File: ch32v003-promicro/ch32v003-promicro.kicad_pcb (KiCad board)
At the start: 2 copper layers, 17.8 x 33 mm, 24 parts, among them J1 USB2.0_C_v3, J2 ProMicro-LeftPin, J3 ProMicro-RightPin, SW1 SW_Push, U1 CH32V003F4P6, U2 AMS1117-3.3, Y1 24M

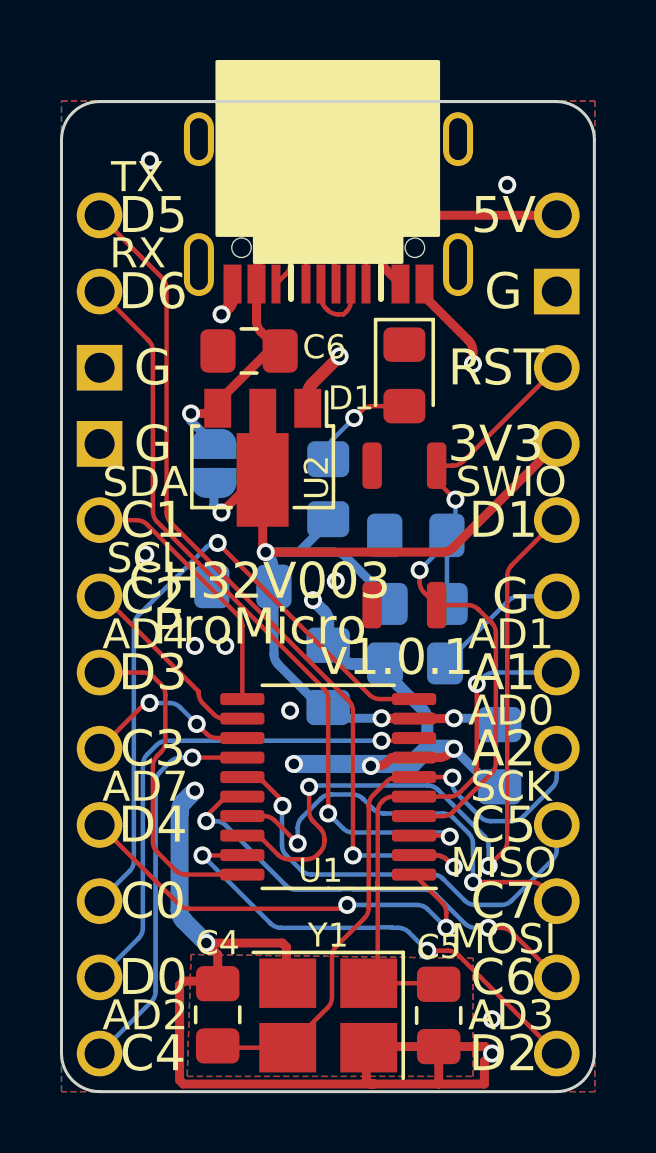
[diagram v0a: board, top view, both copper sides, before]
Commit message: ch32v003promicro/1.1.0
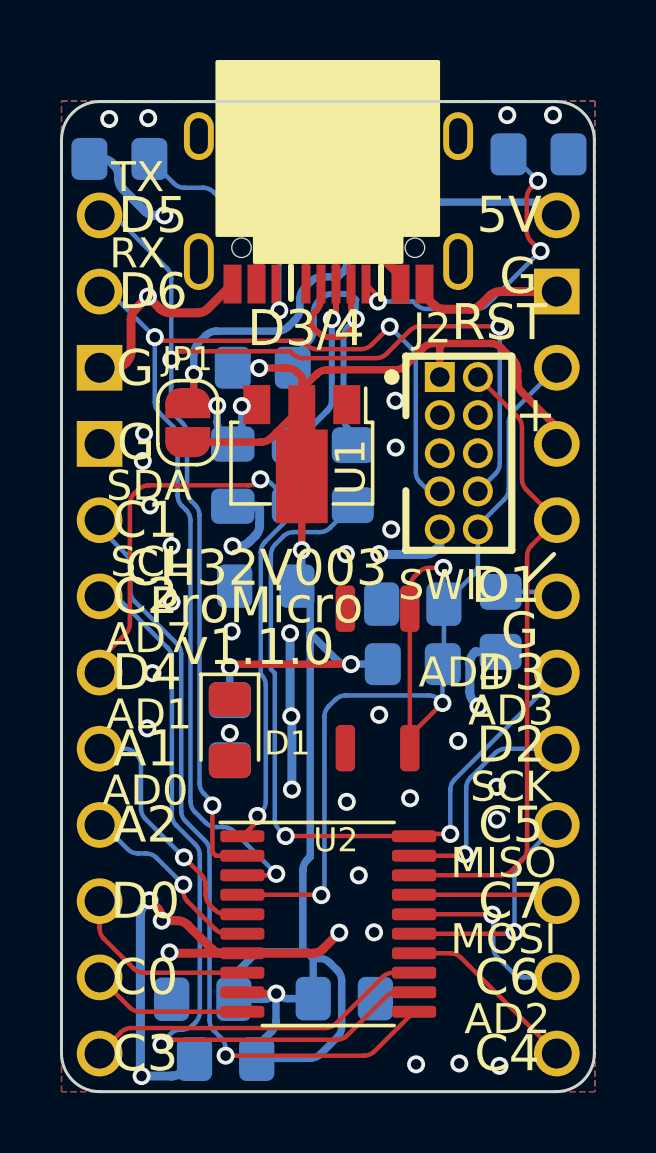
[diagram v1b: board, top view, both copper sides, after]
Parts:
- removed the C4 at (103.0, 92.7)
- removed the C5 at (110.4, 92.7)
- removed the REF** at (104.1, 93.2)
- removed Y1: 24M, $74th:Crystal_SMD_3225-4Pin_3.2x2.5mm_HandSoldering
- added C6: 1u, $74th:Capacitor_0805_2012, B.Cu at (103.3, 94.2)
- added J2: SWD-MCU_Side-10Pin, $74th:SWD_2x05_P1.27mm, F.Cu at (110.4, 71.4)
- added MISC-ACCOUNTTEXT: 74th-text, $74th:74th-text, B.Cu at (111.5, 88.9)
- added MISC-ACCOUNTTEXT: 74th-text, $74th:74th-text, B.Cu at (110.2, 88.8)
- added R1: 10k, $74th:Register_0805_2012, B.Cu at (108.6, 63.2)
- added R2: 54k, $74th:Register_0805_2012, B.Cu at (104.8, 63.2)
- added R5: 1.5k(NC), $74th:Register_0805_2012, B.Cu at (104.5, 71.1)
- added R6: 27.4(NC), $74th:Register_0805_2012, B.Cu at (107.5, 74.7)
- added R7: 27.4(NC), $74th:Register_0805_2012, B.Cu at (105.5, 74.7)
- added U3: CH217K, Package_TO_SOT_SMD:SOT-23-6, B.Cu at (107.1, 65.9)
- C1: renamed from C6; moved to B.Cu
- C2: renamed from C7; value 2.2u -> 10u
- JP1: moved to F.Cu
- R10: renamed from R4; value 200 -> 10k
- moved REF** 18.2 mm to (100.7, 83.2)
- moved D1 13.2 mm to (103.4, 83.2)
- moved C5 12.8 mm to (102.5, 92.2), turned to 180 degrees
- moved C4 10.8 mm to (107.2, 92.2), turned to 0 degrees
- moved R10 8.68 mm to (103.4, 83.2), turned to -90 degrees
- moved G*** 7.45 mm to (110.4, 86.0)
- moved R3 6.04 mm to (113.7, 64.0), turned to 0 degrees
- moved R4 4.97 mm to (99.7, 64.2), turned to 180 degrees
- moved SW1 4.85 mm to (108.3, 81.5)
- moved U2 4.57 mm to (106.7, 89.7), turned to 0 degrees
- moved C1 4.17 mm to (103.5, 74.7), turned to -90 degrees
- moved R8 3.17 mm to (112.4, 79.6), turned to -90 degrees
- moved C3 2.29 mm to (109.5, 79.0)
- moved R9 2.02 mm to (109.5, 81.0)
- moved JP1 1.61 mm to (102.0, 73.0)
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- renumbered C1 to C3, C2 to C4, C3 to C5, J2 to J3, J3 to J4, R2 to R4, R5 to R8, R1 to R9, U2 to U1, U1 to U2
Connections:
- net 0/UART_RX renamed /0/UART_RX
- net 14/SPI_MISO renamed /14/SPI_MISO
- net 15/SPI_SCK renamed /15/SPI_SCK
- net 16/SPI_MOSI renamed /16/SPL_MOSI
- net 1/UART_TX renamed /1/UART_TX
- net 20/A2 renamed /20/A2
- net 21/A3 renamed /21/A3
- net 2/I2C_SDA renamed /2/I2C_SDA
- net 3/I2C_SCL renamed /3/I2C_SCL
- net RST renamed /RST
- J1 pad 1: +5V -> Net-(J1-VBUS)
- J1 pad 2: unconnected-(J1-D--Pad2) -> /USB_D-
- J1 pad 3: unconnected-(J1-D+-Pad3) -> /USB_D+
- J3 pad 10: 7 -> /7
- J3 pad 11: 8/A8 -> /8/A8
- J3 pad 12: 9/A9 -> /9/A9
- J3 pad 7: 4/A6 -> /4/A6
- J3 pad 8: 5 -> /5
- J3 pad 9: 6/A7 -> /6/A7
- J4 pad 1: 10/A10 -> /10/A10
- J4 pad 5: 18/A0 -> /18/A0
- J4 pad 6: 19/A1 -> /19/A1
- U2 pad 1: 6/A7 -> /4/A6
- U2 pad 10: 7 -> /8/A8
- U2 pad 13: 5 -> /9/A9
- U2 pad 14: 9/A9 -> /10/A10
- U2 pad 19: 10/A10 -> /18/A0
- U2 pad 20: 4/A6 -> /19/A1
- U2 pad 5: 19/A1 -> /5
- U2 pad 6: 18/A0 -> /6/A7
- U2 pad 8: 8/A8 -> /7
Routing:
- net /19/A1: track 0.00 -> 25.1 mm, vias 0 -> 2
- net VCC: track 38.8 -> 62.4 mm, vias 4 -> 5
- net /4/A6: track 0.00 -> 23.2 mm, vias 0 -> 2
- net 7: track 22.3 -> 0.00 mm, vias 1 -> 0
- net 18/A0: track 20.6 -> 0.00 mm, vias 1 -> 0
- net /3/I2C_SCL: track 6.55 -> 25.8 mm, vias 0 -> 1
- net 19/A1: track 18.6 -> 0.00 mm, vias 1 -> 0
- net /2/I2C_SDA: track 8.73 -> 26.0 mm, vias 0 -> 1
- net 8/A8: track 17.1 -> 0.00 mm, vias 1 -> 0
- net 10/A10: track 15.8 -> 0.00 mm, vias 2 -> 0
- net 6/A7: track 15.2 -> 0.00 mm, vias 2 -> 0
- net /USB_D-: track 0.00 -> 13.2 mm, vias 0 -> 1
- net 9/A9: track 13.1 -> 0.00 mm, vias 1 -> 0
- net /RST: track 23.5 -> 35.1 mm, vias 2 -> 3
- net /9/A9: track 0.00 -> 11.5 mm
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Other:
- board text added: "+"
- board text added: "D3/4"
- board text added: "USB"
- board text added: "v1.1.0"
- board text removed: "3V3"
- board text removed: "v1.0.0"
- board text removed: "v1.0.1"

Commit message: ch32v003promicro/1.2.0
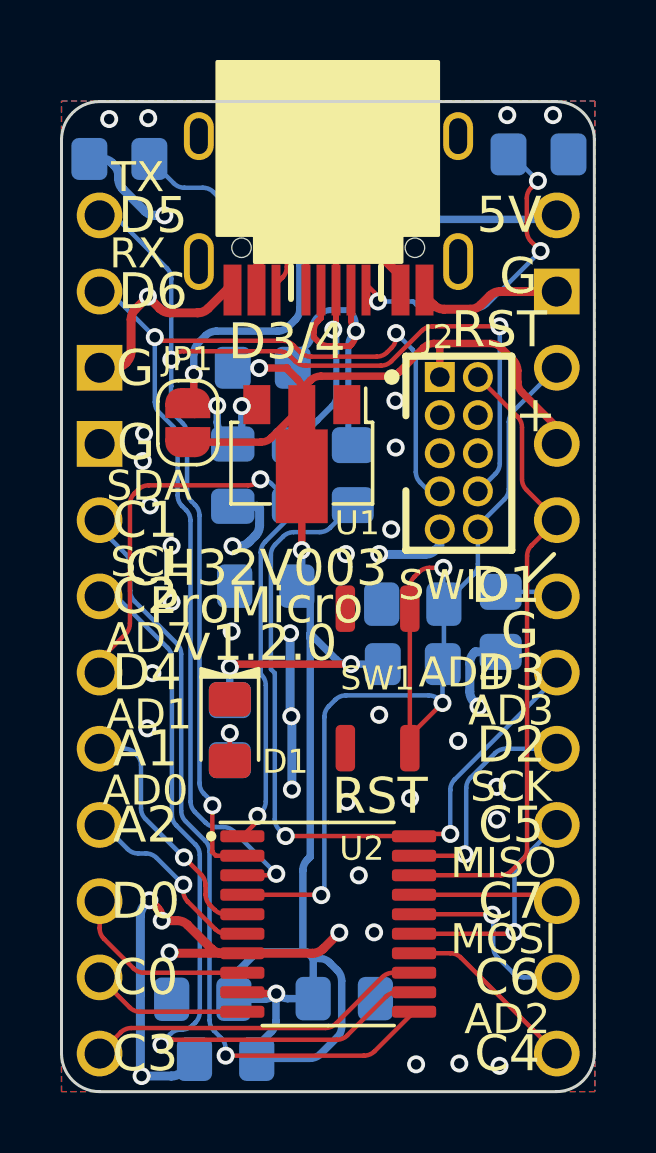
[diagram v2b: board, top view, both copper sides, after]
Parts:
- removed R1: 10k, $74th:Register_0805_2012
- removed R2: 54k, $74th:Register_0805_2012
- C1, C2, C3, C4, C5, C6: footprint $74th:Capacitor_0805_2012 -> 74th:Capacitor_0805_2012
- D1: value LED -> Blue; footprint $74th:LED_0805_2012Metric_Pad1.15x1.40mm_HandSolder -> 74th:LED_0805_2012
- J1: footprint $74th:USB-C-12-Pin-SMD -> 74th:Connector_USB-C-Receptacle_SMT_12-Pin_Simple
- J2: footprint $74th:SWD_2x05_P1.27mm -> 74th:Connector_HalfPinHeader_SWD
- J3: footprint $74th:ProMicro_LIKE_LEFT -> 74th:PinOut_ProMicro-LIKE_LEFT
- J4: footprint $74th:ProMicro_LIKE_RIGHT -> 74th:PinOut_ProMicro-LIKE_RIGHT
- R10, R3, R4, R5, R6, R7, R8, R9: footprint $74th:Register_0805_2012 -> 74th:Register_0805_2012
- SW1: footprint $74th:SKRPABE010 -> 74th:PushButton_SKRPABE010
- U1: footprint Package_TO_SOT_SMD:SOT-89-3 -> 74th:Package_SOT-89-3
- U2: footprint Package_SO:TSSOP-20_4.4x6.5mm_P0.65mm -> 74th:Package_TSSOP-20_4.4x6.5mm_P0.65mm
- U3: value CH217K -> CH213K; footprint Package_TO_SOT_SMD:SOT-23-6 -> 74th:Package_SOT-23
- moved MISC-ACCOUNTTEXT 0.23 mm to (110.5, 88.8)
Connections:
- U3 pad 1: +5V -> GND
- U3 pad 2: GND -> +5V
- U3 pad 3: unconnected-(U3-FLAG#-Pad3) -> Net-(J1-VBUS)
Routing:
- net GND: track 50.1 -> 44.8 mm, vias 43 -> 46
- net Net-(U3-EN#): track 4.06 -> 0.00 mm
- net Net-(U3-ISET): track 4.06 -> 0.00 mm
- net Net-(J1-VBUS): track 9.93 -> 8.08 mm
- net +5V: track 21.0 -> 19.3 mm
- net Net-(J1-CC2): track 8.30 -> 7.20 mm
- net /USB_D-: track 13.2 -> 12.2 mm
- net VCC: track 62.4 -> 61.6 mm
- net /3/I2C_SCL: track 25.8 -> 25.2 mm
- net /5: track 8.40 -> 7.84 mm
- net /6/A7: track 6.28 -> 5.74 mm
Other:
- board text added: "v1.2.0"
- board text removed: "v1.1.0"

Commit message: ch32v003promicto/1.3.0
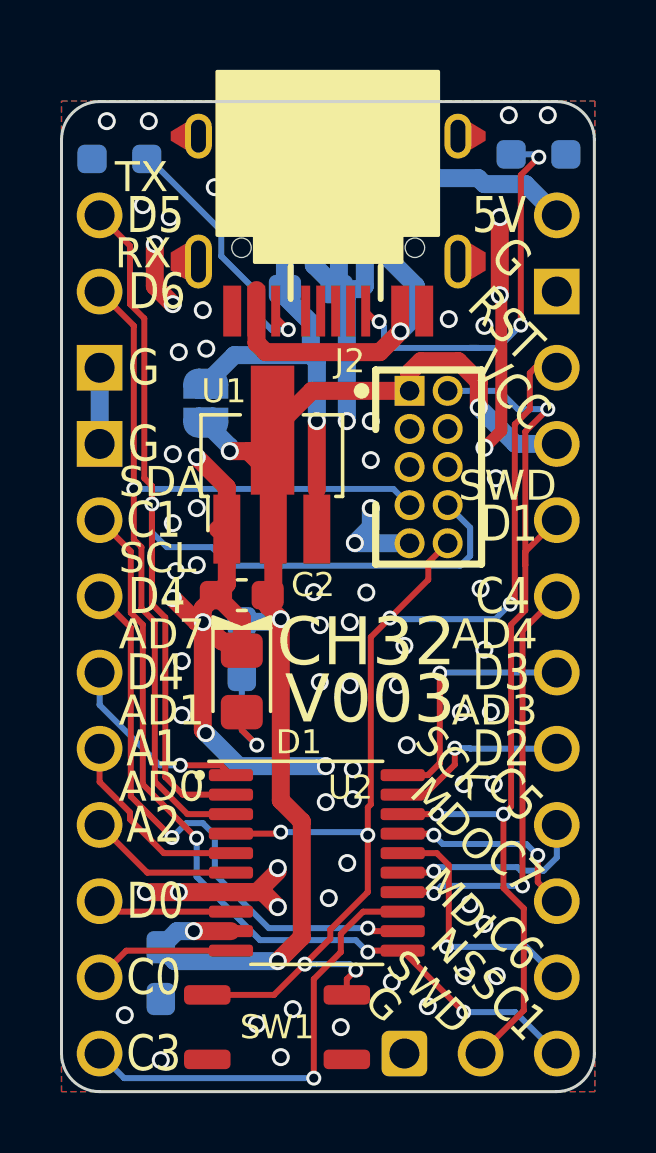
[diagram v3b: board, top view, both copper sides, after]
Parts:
- removed C3, C5: 100n, 74th:Capacitor_0805_2012
- removed C6: 1u, 74th:Capacitor_0805_2012
- removed R5: 1.5k(NC), 74th:Register_0805_2012
- removed R6, R7: 27.4(NC), 74th:Register_0805_2012
- removed R8: 0, 74th:Register_0805_2012
- removed R9: 10k, 74th:Register_0805_2012
- added J5: SWD, 74th:PinOut_Pin_2_2GND, F.Cu at (111.8, 94.0)
- C1, C4: footprint 74th:Capacitor_0805_2012 -> 74th:Capacitor_0603_1608
- C2: footprint 74th:Capacitor_0805_2012 -> 74th:Capacitor_0603_1608; moved to F.Cu
- JP1: footprint Jumper:SolderJumper-2_P1.3mm_Open_RoundedPad1.0x1.5mm -> 74th:SolderJumper-2; moved to B.Cu
- R10, R3, R4: footprint 74th:Register_0805_2012 -> 74th:Register_0603_1608
- SW1: footprint 74th:PushButton_SKRPABE010 -> 74th:Switch_SKRPABE010
- moved SW1 12.1 mm to (105.0, 93.1), turned to 180 degrees
- moved G*** 7.93 mm to (107.4, 78.6)
- moved C1 6.69 mm to (106.0, 68.5), turned to 0 degrees
- moved C4 6.19 mm to (101.1, 91.2), turned to -90 degrees
- moved R10 2.73 mm to (103.8, 80.5)
- moved U2 2.07 mm to (106.3, 87.6)
- moved D1 1.67 mm to (103.8, 81.6)
- moved U3 1.62 mm to (106.7, 64.4), turned to 0 degrees
- moved J2 1.11 mm to (109.4, 71.9)
- moved U1 1.03 mm to (104.8, 74.0), turned to 90 degrees
- moved JP1 0.88 mm to (102.6, 72.3)
- moved C2 0.76 mm to (103.9, 78.7)
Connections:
- net /0/UART_RX renamed /PD6
- net /14/SPI_MISO renamed /PC7
- net /15/SPI_SCK renamed /PC5
- net /16/SPL_MOSI renamed /PC6
- net /18/A0 renamed /PD2
- net /19/A1 renamed /PD3
- net /1/UART_TX renamed /PD5
- net /21/A3 renamed /PD1
- net /3/I2C_SCL renamed /PC2
- net /4/A6 renamed /PD4
- net /5 renamed /PA1
- net /6/A7 renamed /PA2
- net /7 renamed /PD0
- net /8/A8 renamed /PC0
- net /9/A9 renamed /PC3
- J1 pad 2: /USB_D- -> unconnected-(J1-D--Pad2)
- J1 pad 3: /USB_D+ -> unconnected-(J1-D+-Pad3)_1
- J3 pad 5: /2/I2C_SDA -> /PC1
- J4 pad 1: /10/A10 -> /PC1
- J4 pad 7: /20/A2 -> /PC4
- U2 pad 11: /2/I2C_SDA -> /PC1
- U2 pad 14: /10/A10 -> /PC4
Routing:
- net /PC1: track 0.00 -> 27.7 mm, vias 0 -> 3
- net /2/I2C_SDA: track 26.0 -> 0.00 mm, vias 1 -> 0
- net VCC: track 61.6 -> 42.4 mm
- net /PD4: track 23.2 -> 6.43 mm, vias 2 -> 1
- net /PD3: track 25.1 -> 8.31 mm, vias 2 -> 1
- net /PC4: track 0.00 -> 15.0 mm, vias 0 -> 2
- net GND: track 44.8 -> 59.0 mm, vias 46 -> 82
- net /USB_D-: track 12.2 -> 0.00 mm, vias 1 -> 0
- net /PD1: track 21.4 -> 32.3 mm, vias 0 -> 3
- net /USB_D+: track 9.03 -> 0.00 mm, vias 1 -> 0
- net /PD6: track 37.5 -> 29.5 mm, vias 3 -> 1
- net +5V: track 19.3 -> 27.0 mm, vias 3 -> 1
- net /10/A10: track 6.12 -> 0.00 mm
- net /PC2: track 25.2 -> 19.2 mm, vias 1 -> 2
- net Net-(J1-VBUS): track 8.08 -> 13.4 mm
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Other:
- board text added: "CH32"
- board text added: "MDI"
- board text added: "MDO"
- board text added: "NSS"
- board text added: "SWD"
- board text added: "V003"
- board text added: "VCC"
- board text added: "VCC=5V"
- board text added: "v${REVISION}"
- board text removed: "+"
- board text removed: "AD2"
- board text removed: "C2"
- board text removed: "D3/4"
- board text removed: "MISO"
- board text removed: "MOSI"
- board text removed: "SWIO"
- board text removed: "USB"
- board text removed: "v1.2.0"
